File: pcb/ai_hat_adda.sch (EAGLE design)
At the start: 48 parts, among them J1 1X03ST, J2 1X03ST, J3 1X03ST, J4 1X02ST, K1 2X20-RPI, U1 24LC32A, U2 ADS1115, U3 MCP4725, U4 MCP4725

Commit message: updating
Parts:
- K1: value 2X20-RPI -> 2X20-RPI-ALT; device Ai_Connectors:2X20-RPI -> Ai_Connectors:2X20-RPI-ALT
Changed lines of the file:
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@@
 </classes>
 <parts>
-<part name="K1" library="Ai_Connectors" deviceset="2X20-RPI" device=""/>
+<part name="K1" library="Ai_Connectors" deviceset="2X20-RPI" device="-ALT" value="2X20-RPI-ALT"/>
 <part name="U1" library="Ai_IC" deviceset="24LC32A" device=""/>
 <part name="GND10" library="Ai_Power" deviceset="GND" device=""/>

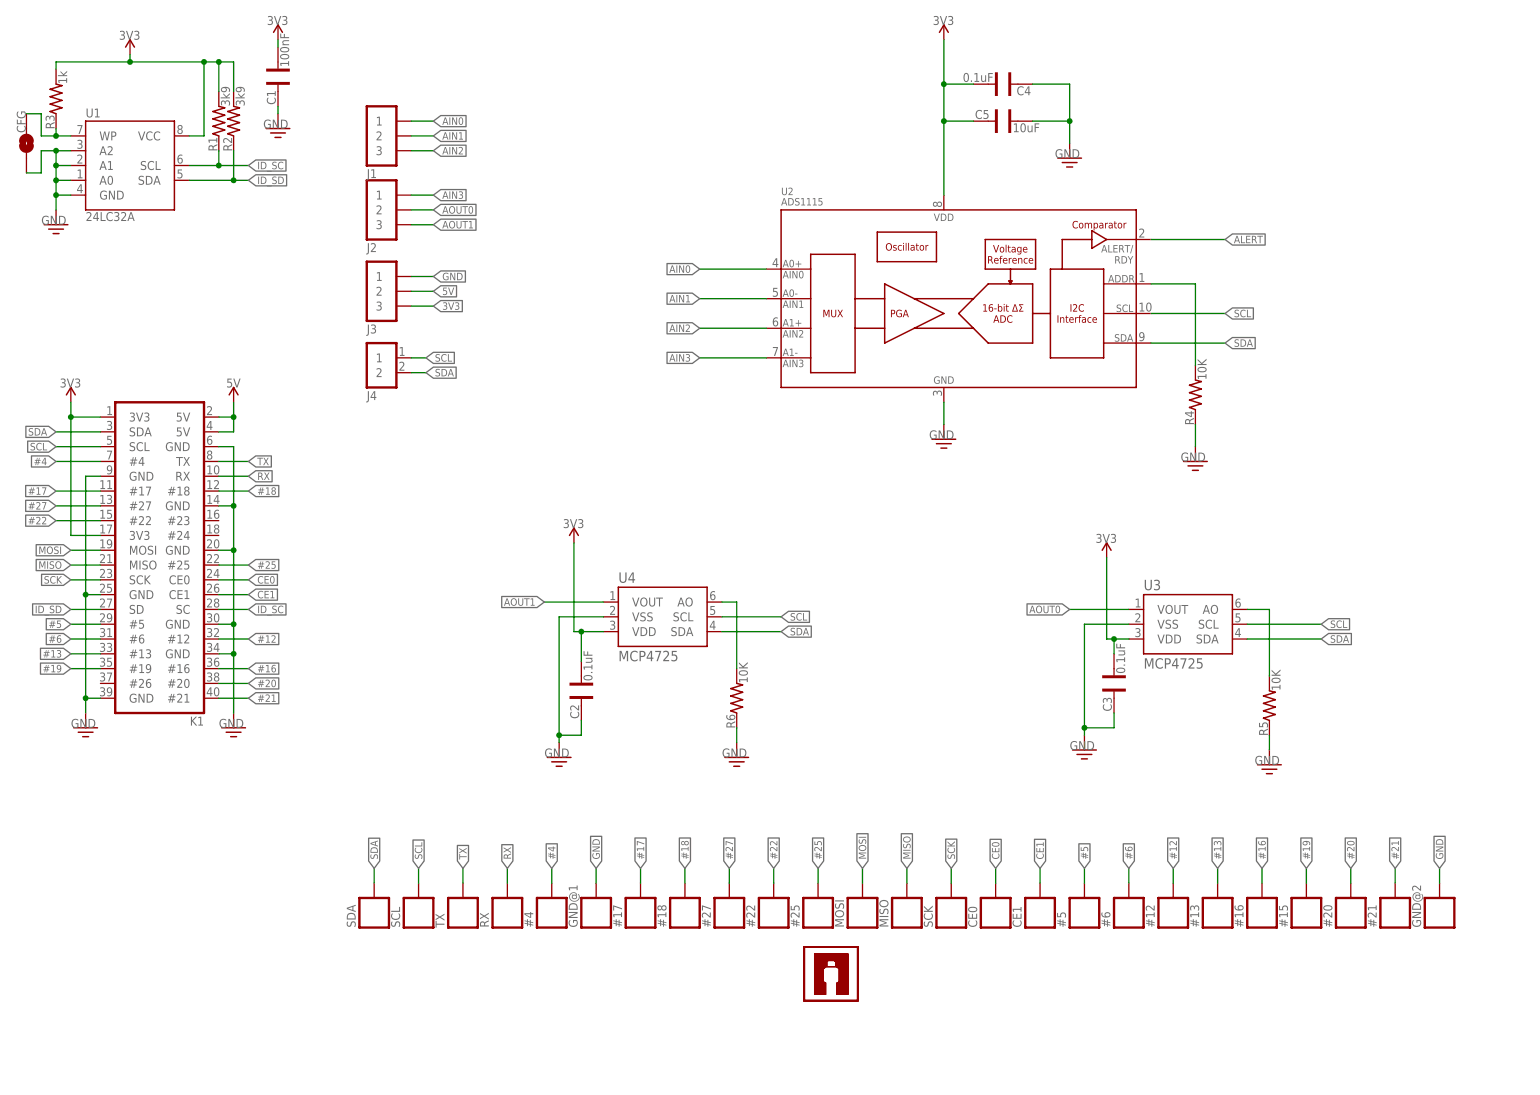
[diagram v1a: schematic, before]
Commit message: updating
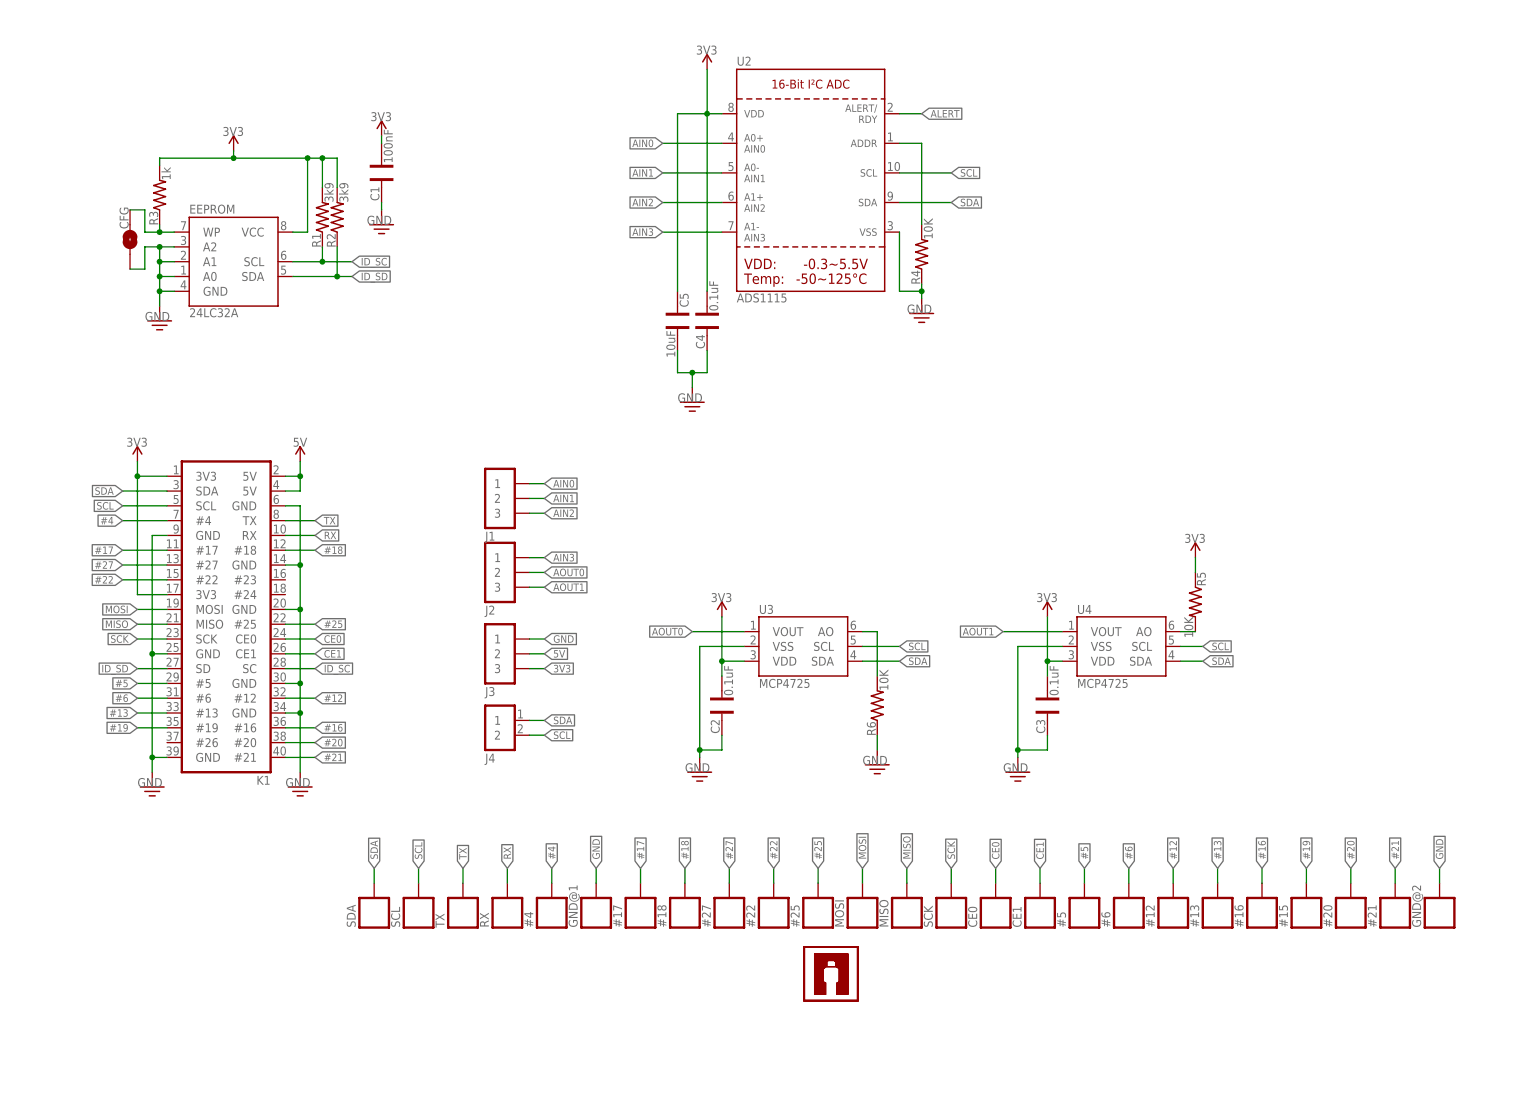
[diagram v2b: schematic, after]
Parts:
- removed U1: 24LC32A, Ai_IC:24LC32A
- added EEPROM: 24LC32A, Ai_IC:24LC32A
- U3, U4: device SparkFun-AnalogIC:MCP4725SOT-23 -> Ai_IC:MCP4725SOT-23
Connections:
- net 3V3: now also EEPROM.VCC, R5.1; no longer U1.VCC
- net GND: now also EEPROM.A0, EEPROM.A1, EEPROM.A2, EEPROM.GND; no longer R5.1, U1.A0, U1.A1, U1.A2, U1.GND
- net ID_SC: now also EEPROM.SCL; no longer U1.SCL
- net ID_SD: now also EEPROM.SDA; no longer U1.SDA
- net N$2: now also U3.AO; no longer U4.AO
- net N$3: now also EEPROM.WP; no longer U1.WP
- net N$4: now also U4.AO; no longer U3.AO
- net SCL: now also J4.2; no longer J4.1
- net SDA: now also J4.1; no longer J4.2
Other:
- moved on the sheet: C1, C2, C3, C4, C5, CFG, J1, J2, J3, J4, K1, R1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

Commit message: updating
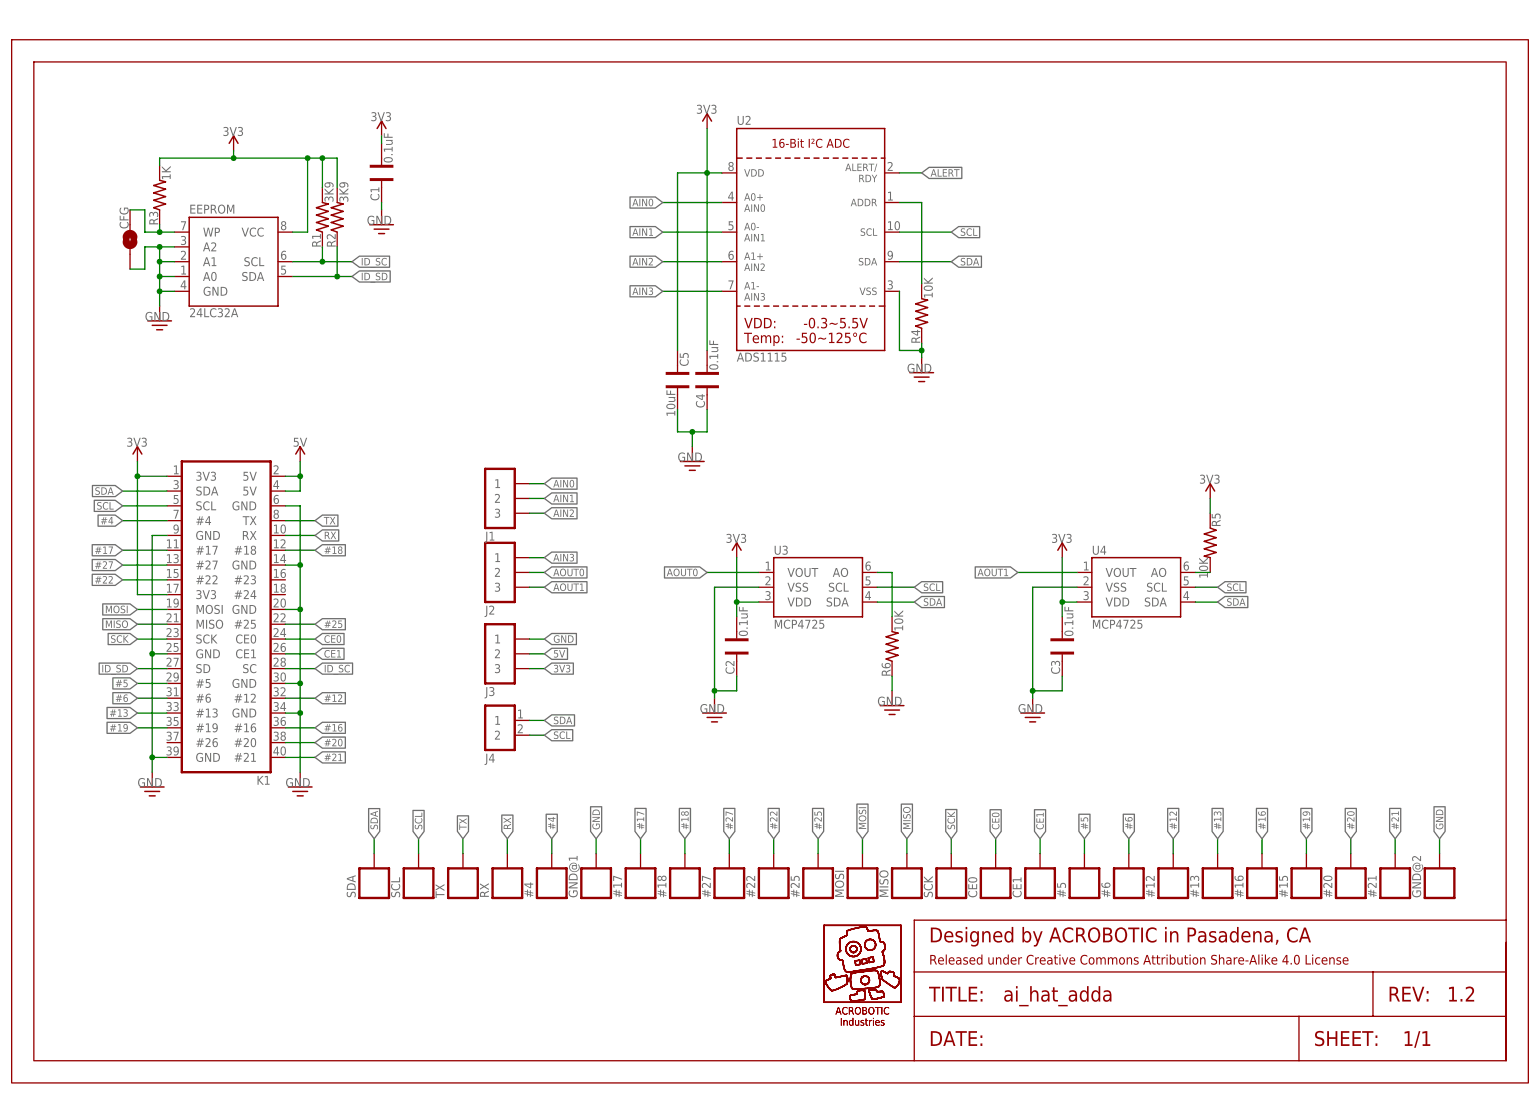
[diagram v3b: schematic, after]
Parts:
- added FRAME1: FRAME-LETTER, Ai_Miscellany:FRAME-LETTER
- C1: value 100nF -> 0.1uF
- R1, R2: value 3k9 -> 3K9
- R3: value 1k -> 1K
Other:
- moved on the sheet: #12, #13, #15, #16, #17, #18, #20, #21, #22, #25, #27, #4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
